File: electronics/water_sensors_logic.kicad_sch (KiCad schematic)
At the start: 3 parts, among them J10 water_sensor_conn, Q1 BF245B

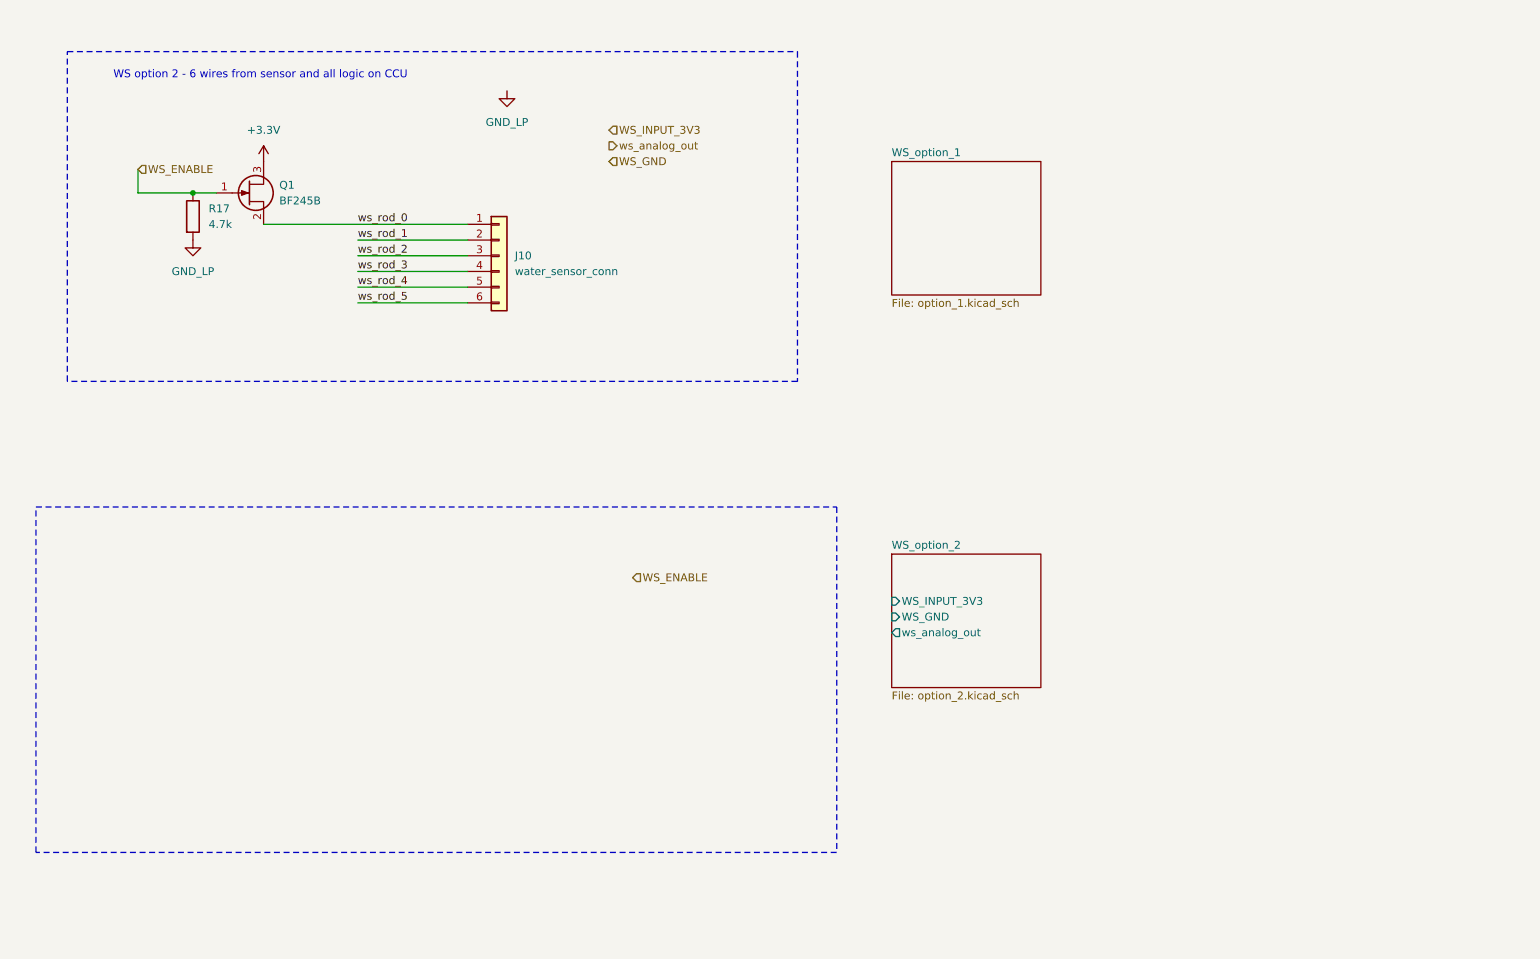
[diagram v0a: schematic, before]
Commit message: flight back. different layout. start analog ui
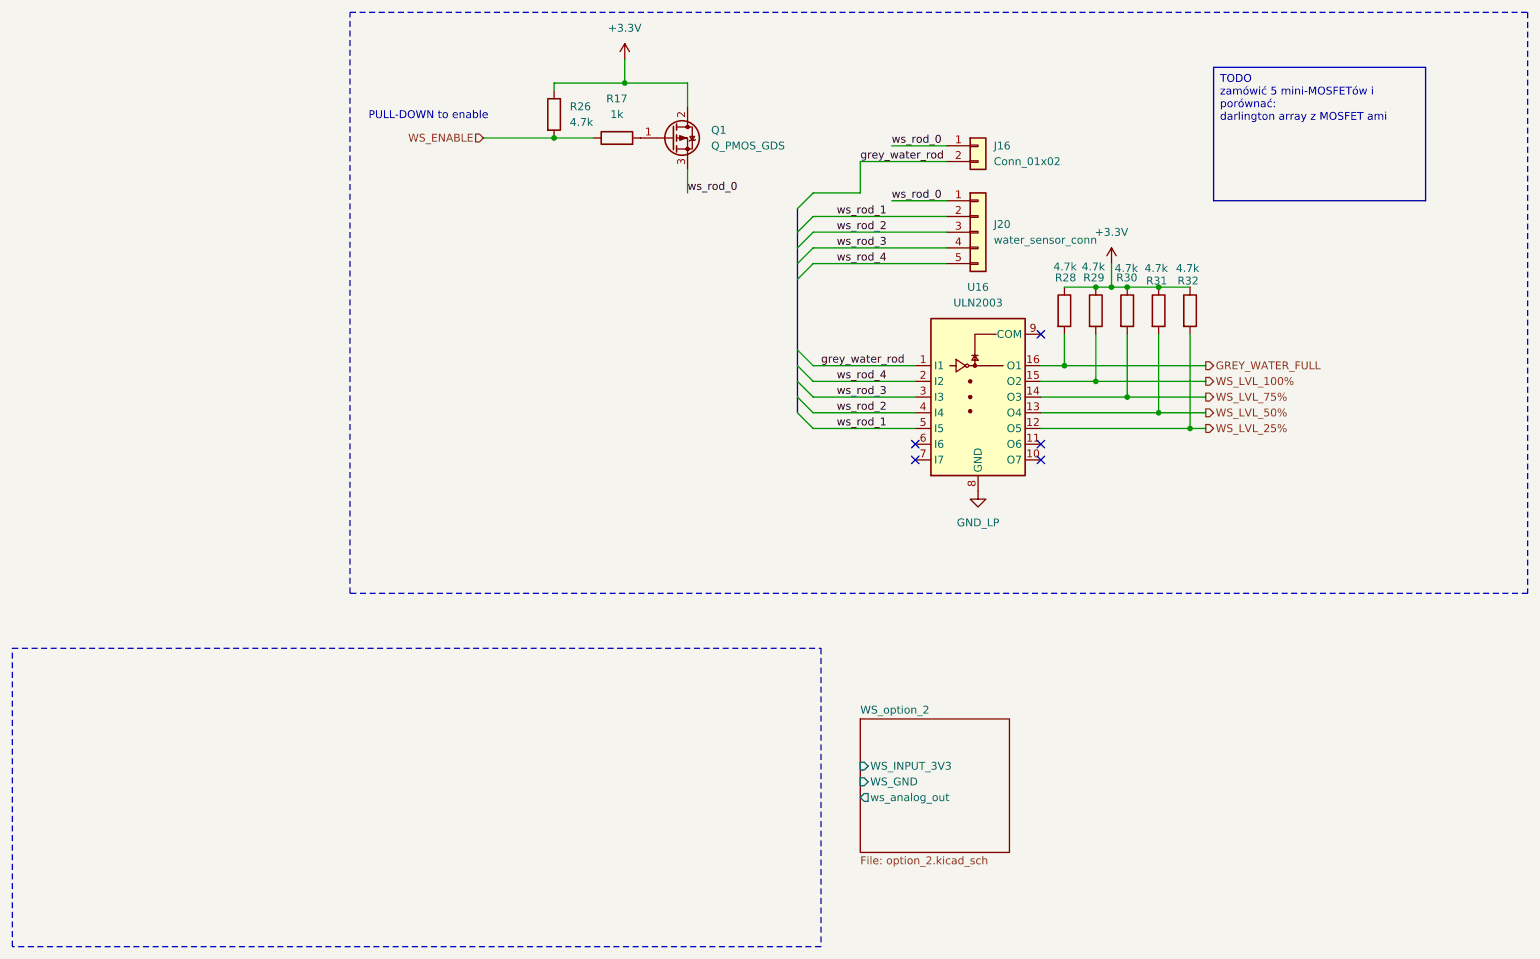
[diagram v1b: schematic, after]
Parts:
- removed J10: water_sensor_conn, TerminalBlock:TerminalBlock_Xinya_XY308-2.54-6P_1x06_P2.54mm_Horizontal, symbol Connector_Generic:Conn_01x06
- removed Q1: BF245B, Package_TO_SOT_THT:TO-92_Inline, symbol Transistor_FET:BF245B
- added J16: Conn_01x02, TerminalBlock:TerminalBlock_Xinya_XY308-2.54-2P_1x02_P2.54mm_Horizontal, symbol Connector_Generic:Conn_01x02
- added J20: water_sensor_conn, TerminalBlock:TerminalBlock_Xinya_XY308-2.54-5P_1x05_P2.54mm_Horizontal, symbol Connector_Generic:Conn_01x05
- added Q1: Q_PMOS_GDS, Package_TO_SOT_SMD:SOT-23_Handsoldering, symbol Device:Q_PMOS_GDS
- added R26, R28, R29, R30, R31, R32: 4.7k, Resistor_SMD:R_0805_2012Metric_Pad1.20x1.40mm_HandSolder, symbol Device:R
- added U16: ULN2003, Package_SO:SO-16_3.9x9.9mm_P1.27mm, symbol Transistor_Array:ULN2003
- R17: value 4.7k -> 1k; footprint (none) -> Resistor_SMD:R_0805_2012Metric_Pad1.20x1.40mm_HandSolder
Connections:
- net +3.3V: now also Q1.2 (D), R26.1, R28.1, R29.1, R30.1, R31.1, R32.1
- net GND_LP: now also U16.8 (GND); no longer R17.2
- net WS_ENABLE: now also R26.2
- net ws_rod_0: now also J16.1 (Pin_1), J20.1 (Pin_1), Q1.3 (S)
- net ws_rod_1: now also J20.2 (Pin_2), U16.5 (I5)
- net ws_rod_2: now also J20.3 (Pin_3), U16.4 (I4)
- net ws_rod_3: now also J20.4 (Pin_4), U16.3 (I3)
- net ws_rod_4: now also J20.5 (Pin_5), U16.2 (I2)
- new net: Q1.1 (G), R17.2
- new net GREY_WATER_FULL: R28.2, U16.16 (O1)
- new net WS_LVL_100%: R29.2, U16.15 (O2)
- new net WS_LVL_25%: R32.2, U16.12 (O5)
- new net WS_LVL_50%: R31.2, U16.13 (O4)
- new net WS_LVL_75%: R30.2, U16.14 (O3)
- new net grey_water_rod: J16.2 (Pin_2), U16.1 (I1)
- no-connect marks 0 -> 5
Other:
- removed sheet WS_option_1
- note added: "PULL-DOWN to enable"
- note removed: "WS option 2 - 6 wires from sensor and all logic on CCU"
- moved on the sheet: R17
